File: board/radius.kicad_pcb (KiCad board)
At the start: 2 copper layers, 25.4 x 12.1 mm, 11 parts, among them IC1 STM8S003F3P, P1 CONN_01X04, P2 CONN_01X10, U1 CH340G, U2 LM2931AZ-3.3/5.0, Y1 Crystal

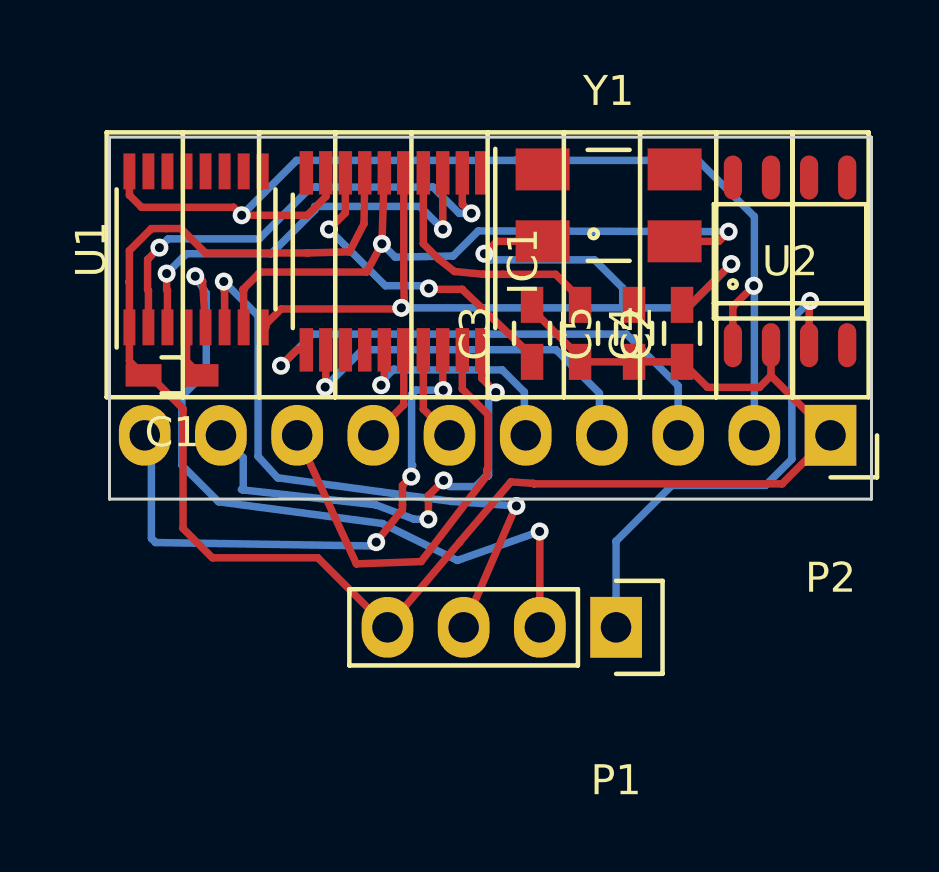
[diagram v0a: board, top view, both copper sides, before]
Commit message: Qualifying layout
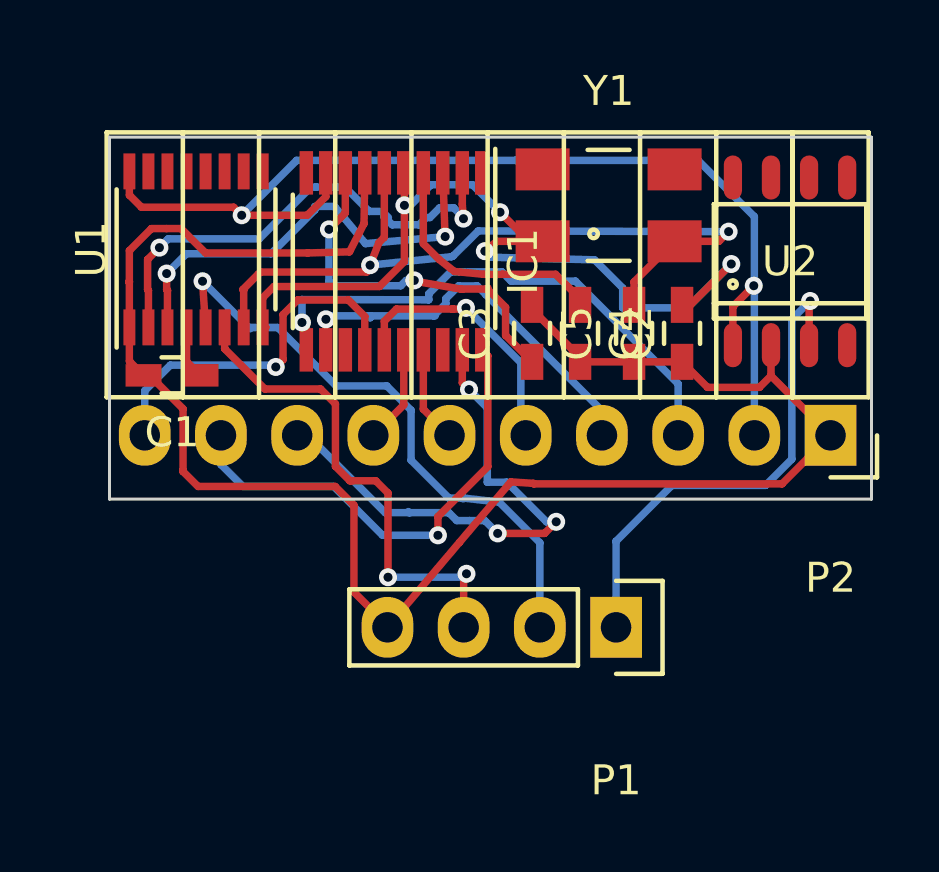
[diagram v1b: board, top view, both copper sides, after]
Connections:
- IC1 pad 14: Net-(IC1-Pad14) -> G3
- IC1 pad 18: G3 -> Net-(IC1-Pad18)
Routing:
- net G3: track 19.0 -> 12.7 mm, vias 3 -> 1
- net D-: track 21.2 -> 16.7 mm
- net D+: track 24.8 -> 20.3 mm, vias 2 -> 1
- net TXD: track 15.0 -> 18.7 mm, vias 0 -> 3
- net XI: track 23.4 -> 26.4 mm
- net XO: track 31.4 -> 29.3 mm, vias 3 -> 4
- net SDA: track 17.1 -> 19.1 mm
- net Net-(C3-Pad1): track 10.8 -> 12.6 mm
- net SCK: track 8.09 -> 9.02 mm
- net SCL: track 12.9 -> 13.6 mm
- net GND: track 59.9 -> 60.6 mm
- net USB_TX: track 15.9 -> 16.6 mm
- net USB_RX: track 14.2 -> 14.8 mm
- net RXD: track 16.5 -> 16.4 mm, vias 3 -> 1
